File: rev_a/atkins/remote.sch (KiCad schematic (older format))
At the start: 17 parts, among them J1 UARTSCREW, J10 Conn_01x04_Female, J11 BME390, J2 UARTPINS, J4 Screw_Terminal_01x04, J5 Conn_01x02_Female, J6 Conn_01x12_Male, J7 Conn_01x16_Female, J8 Screw_Terminal_01x02, J9 SCD30

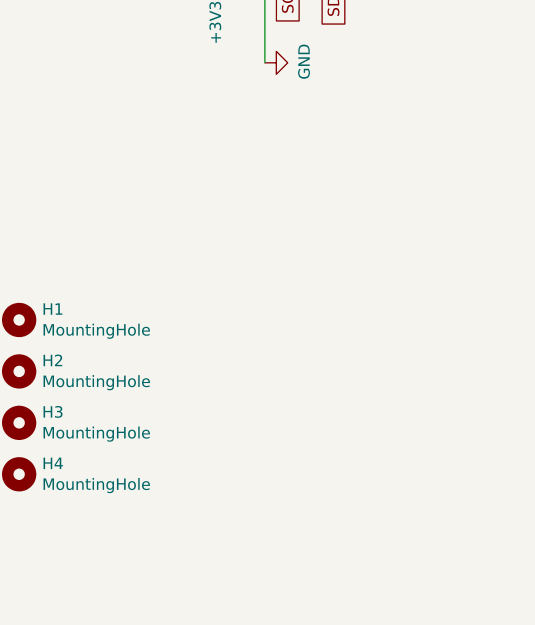
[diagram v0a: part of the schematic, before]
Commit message: update
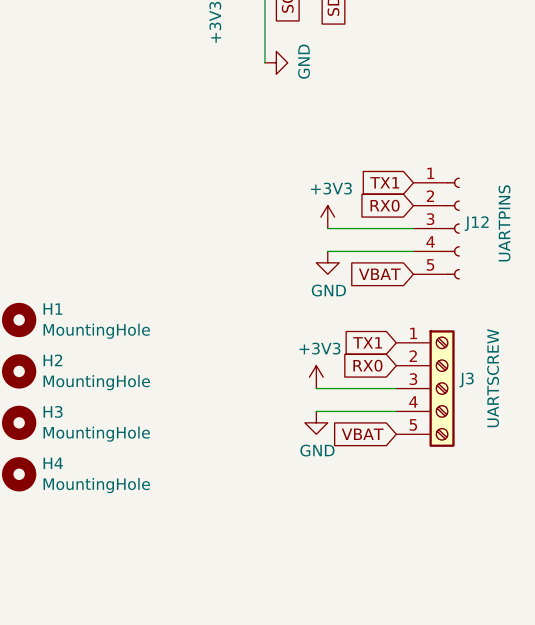
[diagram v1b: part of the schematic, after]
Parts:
- added J12: UARTPINS, Connector_PinSocket_2.54mm:PinSocket_1x05_P2.54mm_Vertical, symbol Connector:Conn_01x05_Female
- added J3: UARTSCREW, TerminalBlock_Phoenix:TerminalBlock_Phoenix_MKDS-1,5-5_1x05_P5.00mm_Horizontal, symbol Connector:Screw_Terminal_01x05
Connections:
- net +3V3: now also J12.3 (Pin_3), J3.3 (Pin_3)
- net GND: now also J12.4 (Pin_4), J3.4 (Pin_4)
- net RX0: now also J12.2 (Pin_2), J3.2 (Pin_2)
- net TX1: now also J12.1 (Pin_1), J3.1 (Pin_1)
- net VBAT: now also J12.5 (Pin_5), J3.5 (Pin_5)
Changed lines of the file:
@@
 Text GLabel 4625 1450 0    50   Input ~ 0
 SDA
+$Comp
+L power:+3V3 #PWR0121
+U 1 1 5FC13358
+P 6250 2850
+F 0 "#PWR0121" H 6250 2700 50  0001 C CNN
+F 1 "+3V3" H 6265 3023 50  0000 C CNN
+F 2 "" H 6250 2850 50  0001 C CNN
+F 3 "" H 6250 2850 50  0001 C CNN
+	1    6250 2850
+	1    0    0    -1
+$EndComp
+$Comp
+L power:GND #PWR0122
+U 1 1 5FC1335E
+P 6250 2950
+F 0 "#PWR0122" H 6250 2700 50  0001 C CNN
+F 1 "GND" H 6255 2777 50  0000 C CNN
+F 2 "" H 6250 2950 50  0001 C CNN
+F 3 "" H 6250 2950 50  0001 C CNN
+	1    6250 2950
+	1    0    0    -1
+$EndComp
+Wire Wire Line
+	6625 2850 6250 2850
+Wire Wire Line
+	6625 2950 6250 2950
+$Comp
+L Connector:Screw_Terminal_01x05 J3
+U 1 1 5FC13366
+P 6750 3550
+F 0 "J3" H 6830 3592 50  0000 L CNN
+F 1 "UARTSCREW" V 6975 3375 50  0000 L CNN
+F 2 "TerminalBlock_Phoenix:TerminalBlock_Phoenix_MKDS-1,5-5_1x05_P5.00mm_Horizontal" H 6750 3550 50  0001 C CNN
+F 3 "~" H 6750 3550 50  0001 C CNN
+	1    6750 3550
+	1    0    0    -1
+$EndComp
+$Comp
+L Connector:Conn_01x05_Female J12
+U 1 1 5FC1336C
+P 6825 2850
+F 0 "J12" H 6853 2876 50  0000 L CNN
+F 1 "UARTPINS" V 7025 2700 50  0000 L CNN
+F 2 "Connector_PinSocket_2.54mm:PinSocket_1x05_P2.54mm_Vertical" H 6825 2850 50  0001 C CNN
+F 3 "~" H 6825 2850 50  0001 C CNN
+	1    6825 2850
+	1    0    0    -1
+$EndComp
+Text GLabel 6625 3050 0    50   Input ~ 0
+VBAT
+Text GLabel 6550 3750 0    50   Input ~ 0
+VBAT
+$Comp
+L power:GND #PWR0123
+U 1 1 5FC13374
+P 6200 3650
+F 0 "#PWR0123" H 6200 3400 50  0001 C CNN
+F 1 "GND" H 6205 3477 50  0000 C CNN
+F 2 "" H 6200 3650 50  0001 C CNN
+F 3 "" H 6200 3650 50  0001 C CNN
+	1    6200 3650
+	1    0    0    -1
+$EndComp
+Wire Wire Line
+	6550 3650 6200 3650
+$Comp
+L power:+3V3 #PWR0124
+U 1 1 5FC1337B
+P 6200 3550
+F 0 "#PWR0124" H 6200 3400 50  0001 C CNN
+F 1 "+3V3" H 6215 3723 50  0000 C CNN
+F 2 "" H 6200 3550 50  0001 C CNN
+F 3 "" H 6200 3550 50  0001 C CNN
+	1    6200 3550
+	1    0    0    -1
+$EndComp
+Wire Wire Line
+	6550 3550 6200 3550
+Text GLabel 6625 2750 0    50   Input ~ 0
+RX0
+Text GLabel 6625 2650 0    50   Input ~ 0
+TX1
+Text GLabel 6550 3450 0    50   Input ~ 0
+RX0
+Text GLabel 6550 3350 0    50   Input ~ 0
+TX1
 $EndSCHEMATC
